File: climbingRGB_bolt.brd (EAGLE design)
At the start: 31.8 x 15.2 mm, 8 parts

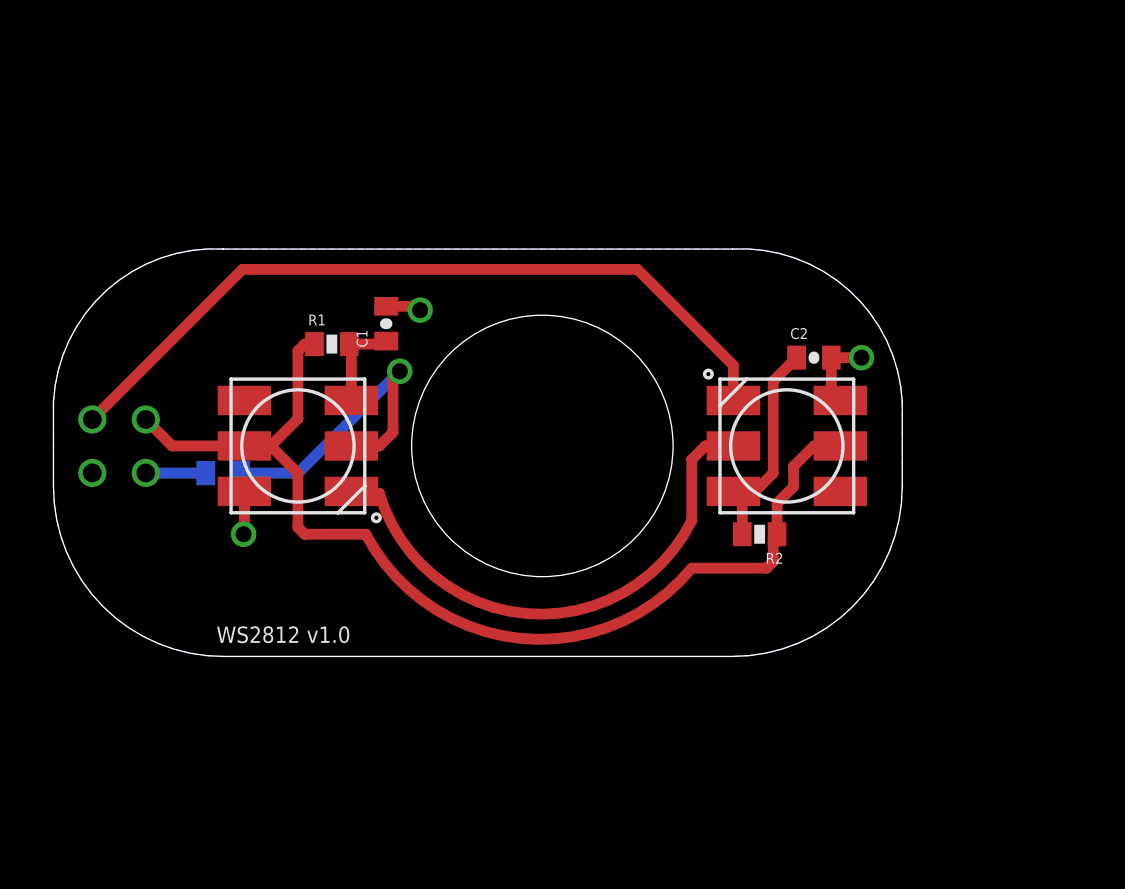
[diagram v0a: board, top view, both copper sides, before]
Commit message: new things!
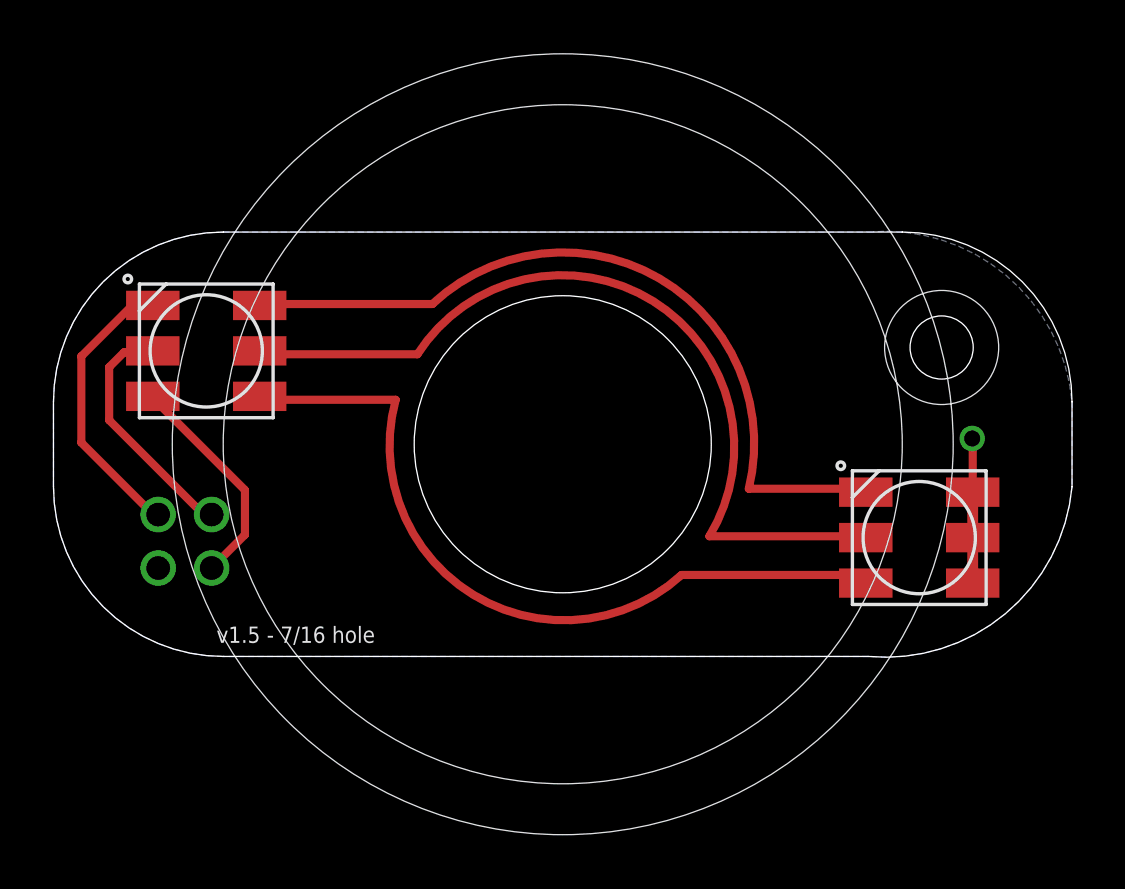
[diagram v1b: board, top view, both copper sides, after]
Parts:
- removed C1, C2: .1uF, SparkFun-Passives:0402-CAP
- removed R1, R2: 150, SparkFun-Passives:0402-RES
- removed R3: 22, SparkFun-Passives:0402-RES
- removed U$2, U$3: WS2812, adafruit:RGBLED5050
- added LED3, LED4: RGBLED5050, adafruit:RGBLED5050
- moved U$1 4.33 mm to (4.88, 4.32)
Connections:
- removed net DI: R3.2, U$2.5
- removed net DODI: U$2.4, U$3.5
- removed net GND: C1.2, C2.2, U$1.P$4, U$2.3, U$3.3
- removed net N$2: U$1.P$1, U$3.4
- removed net VCC2: C2.1, R2.2, U$3.6
- removed net VDD: R1.1, R2.1, U$1.P$2, U$2.2, U$3.2
- new net BLUE: LED4.4, U$1.P$1
- new net GREEN: LED4.6, U$1.P$3
- new net N$5: LED3.6, LED4.1
- new net N$6: LED3.5, LED4.2
- new net RED: LED4.5, U$1.P$2
- net N$1: now also LED3.4, LED4.3; no longer R3.1, U$1.P$3
- net VCC: now also LED3.1, LED3.2, LED3.3, U$1.P$4; no longer C1.1, R1.2, U$2.6
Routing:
- net VDD: track 37.8 -> 0.00 mm
- net N$2: track 29.1 -> 0.00 mm
- net N$5: track 0.00 -> 24.7 mm
- net N$6: track 0.00 -> 24.7 mm
- net N$1: track 2.25 -> 24.6 mm
- net DODI: track 16.9 -> 0.00 mm
- net DI: track 11.7 -> 0.00 mm, vias 1 -> 0
- net BLUE: track 0.00 -> 10.7 mm
- net RED: track 0.00 -> 9.16 mm
- net GREEN: track 0.00 -> 8.37 mm
- net VCC2: track 8.20 -> 0.00 mm
- net GND: track 5.81 -> 0.00 mm, vias 3 -> 0
- net VCC: track 3.57 -> 5.41 mm, vias 0 -> 1
- added copper zone on layer 16, net VCC
- removed copper zone on layer 16, net GND
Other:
- board size 31.8 x 15.2 mm -> 38.1 x 15.9 mm
- board text added: "v1.5 - 7/16 hole"
- board text removed: "WS2812 v1.0"
